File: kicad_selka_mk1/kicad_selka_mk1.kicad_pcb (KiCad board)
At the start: 2 copper layers, 96 x 207.5 mm, 102 parts, among them J1 Conn_01x06_Pin, J10 Conn_01x01_Pin, J11 Conn_01x01_Pin, J12 Conn_01x01_Pin, J13 Conn_01x01_Pin, J14 Conn_01x01_Pin, J15 Conn_01x01_Pin, J16 Conn_01x01_Pin, J17 Conn_01x01_Pin, J18 Conn_01x01_Pin, J19 Conn_01x01_Pin, J2 Conn_01x02_Pin, J20 Conn_01x01_Pin, J21 Conn_01x01_Pin, J22 Conn_01x01_Pin, J23 Conn_01x01_Pin, J24 Conn_01x01_Pin, J25 Conn_01x01_Pin, J26 Conn_01x01_Pin, J27 Conn_01x01_Pin, J28 Conn_01x01_Pin, J3 Conn_01x01_Pin, J4 Conn_01x01_Pin, J5 Conn_01x01_Pin, J6 Conn_01x01_Pin, J7 Conn_01x01_Pin, J8 Conn_01x01_Pin, J9 Conn_01x01_Pin, U1 ATtiny861A-S

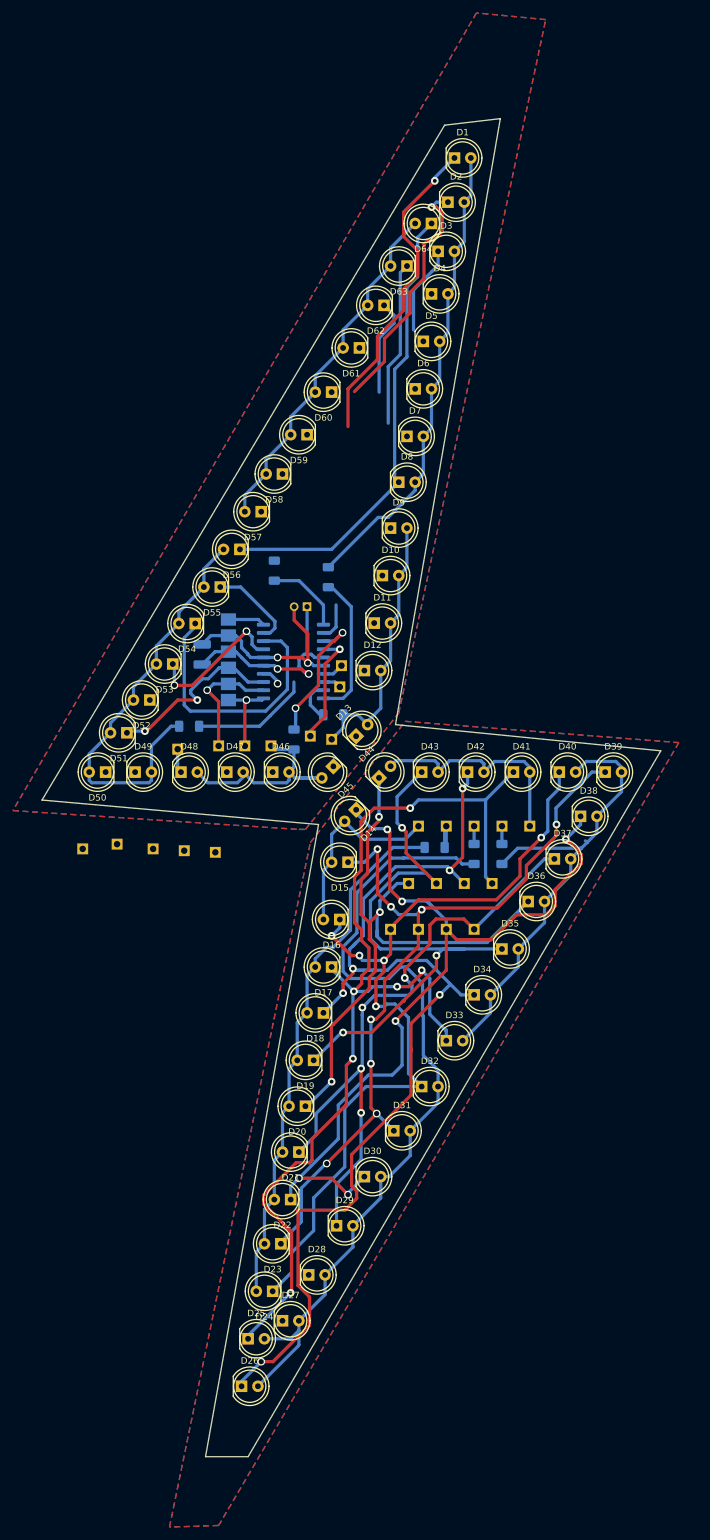
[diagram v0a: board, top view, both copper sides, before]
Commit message: Selkäsalama 90% done
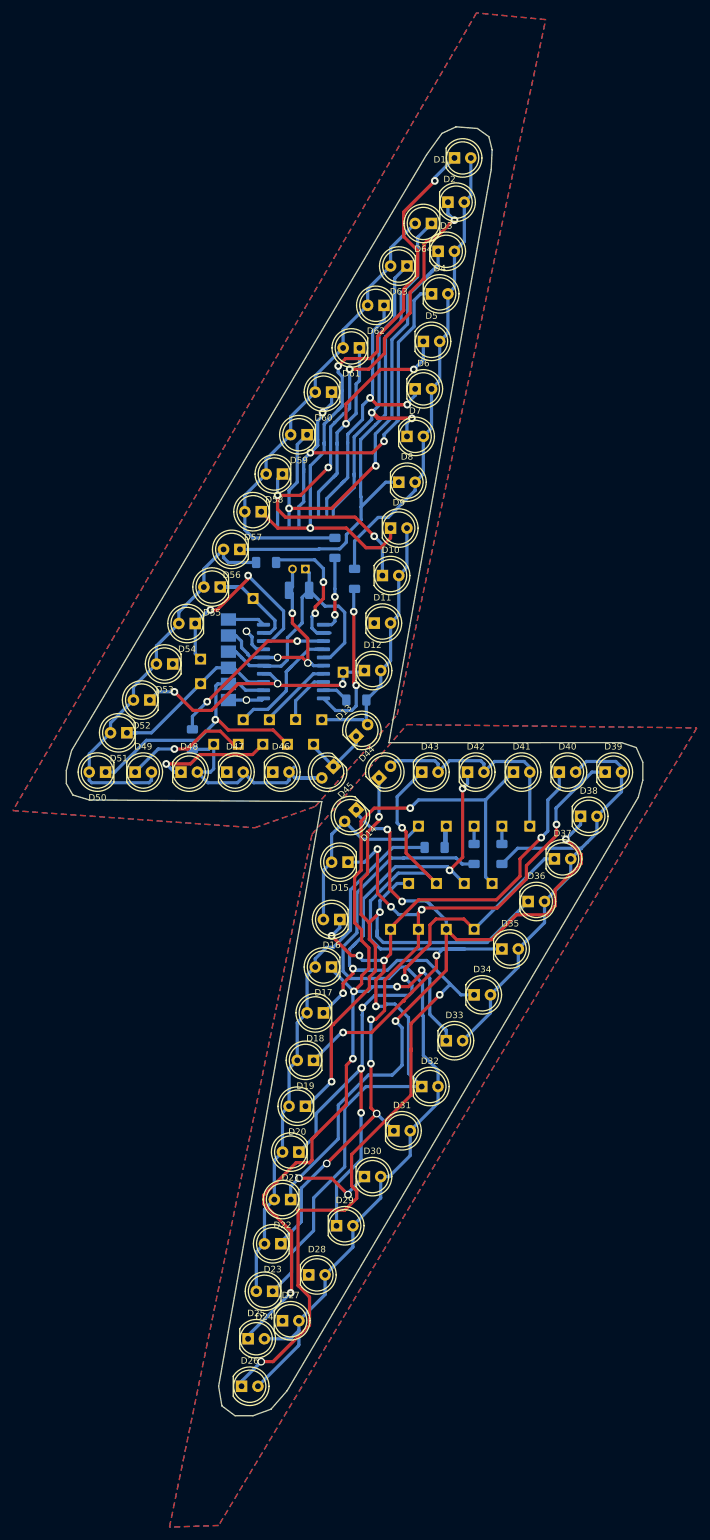
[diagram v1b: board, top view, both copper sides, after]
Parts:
- moved J25 47.0 mm to (113.3, 116.1)
- moved J19 37.1 mm to (127.3, 127.5)
- moved J23 31.5 mm to (105.2, 125.5)
- moved J21 29.7 mm to (122.7, 138.7)
- moved R7 28.1 mm to (115.3, 110.5)
- moved J17 26.3 mm to (105.2, 129.3)
- moved C1 18.0 mm to (120.4, 114.8), turned to 180 degrees
- moved R6 15.7 mm to (103.9, 137.9)
- moved J7 14.0 mm to (115.8, 134.9)
- moved J27 13.2 mm to (114.8, 138.7)
- moved J9 10.7 mm to (111.8, 134.9)
- moved J15 10.7 mm to (118.6, 138.7)
- moved R8 10.0 mm to (126.0, 108.2)
- moved J11 8.89 mm to (107.2, 138.7)
- moved J5 8.52 mm to (119.9, 134.8)
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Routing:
- net Net-(D12-K): track 3.04 -> 105.9 mm, vias 1 -> 6
- net Net-(D10-K): track 57.7 -> 142.3 mm, vias 2 -> 6
- net Net-(D11-K): track 42.1 -> 102.2 mm
- net Net-(D1-K): track 63.2 -> 122.5 mm, vias 2 -> 5
- net Net-(D13-K): track 22.5 -> 66.6 mm, vias 2 -> 3
- net Net-(D47-K): track 39.4 -> 77.1 mm, vias 0 -> 2
- net Net-(D46-K): track 56.8 -> 84.0 mm, vias 0 -> 4
- net Net-(D48-K): track 81.3 -> 106.1 mm, vias 0 -> 1
- net Net-(D20-K): track 154.1 -> 171.4 mm
- net +5V: track 34.6 -> 43.1 mm, vias 2 -> 0
- net Net-(J7-Pin_1): track 3.32 -> 11.5 mm
- net Net-(J5-Pin_1): track 2.86 -> 8.43 mm
- net Net-(U1-PA5): track 23.5 -> 27.4 mm
- net Net-(D45-A): track 35.6 -> 39.3 mm
- net Net-(D10-A): track 43.9 -> 40.6 mm
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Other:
- board size 96 x 207.5 mm -> 89.4 x 199.9 mm
- board text removed: "${REFERENCE}"
